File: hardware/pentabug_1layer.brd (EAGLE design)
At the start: 33 x 82.9 mm, 17 parts, among them IC1 ATMEGA88

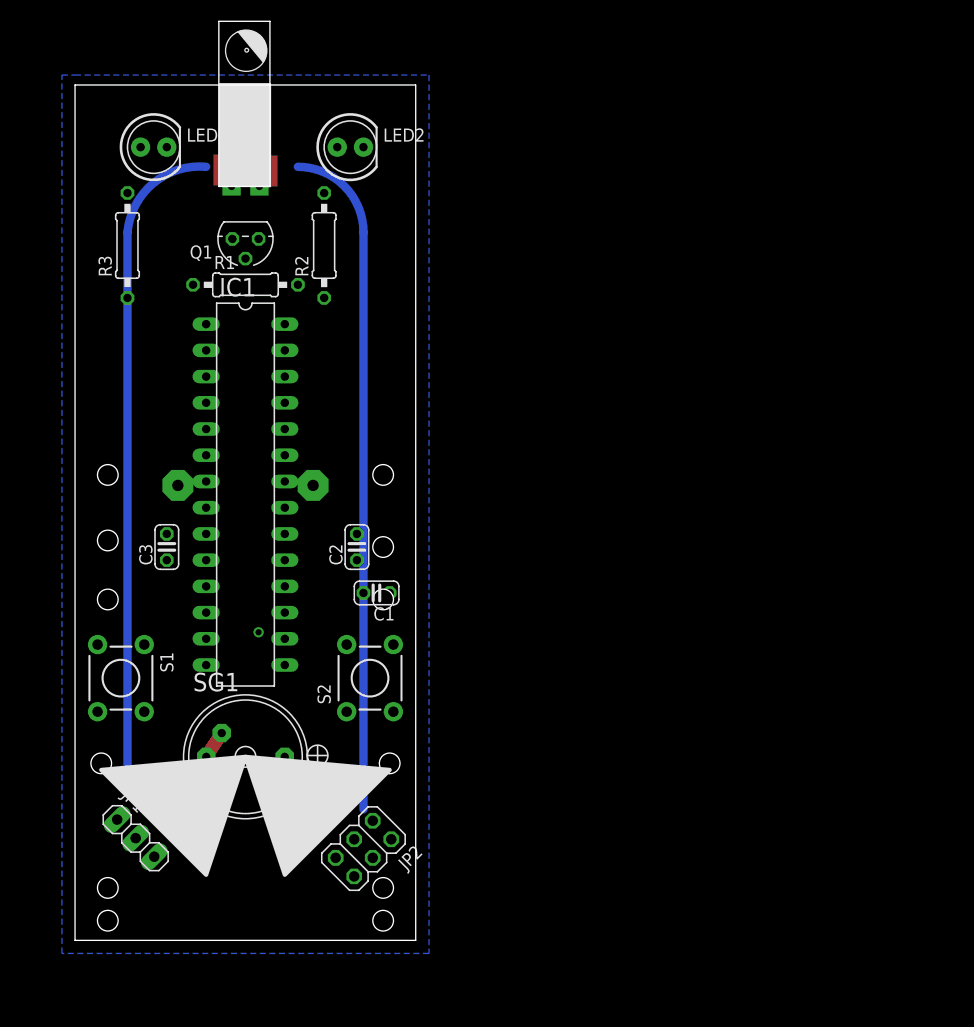
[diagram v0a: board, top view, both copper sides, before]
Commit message: made editable with eagle freeware!!
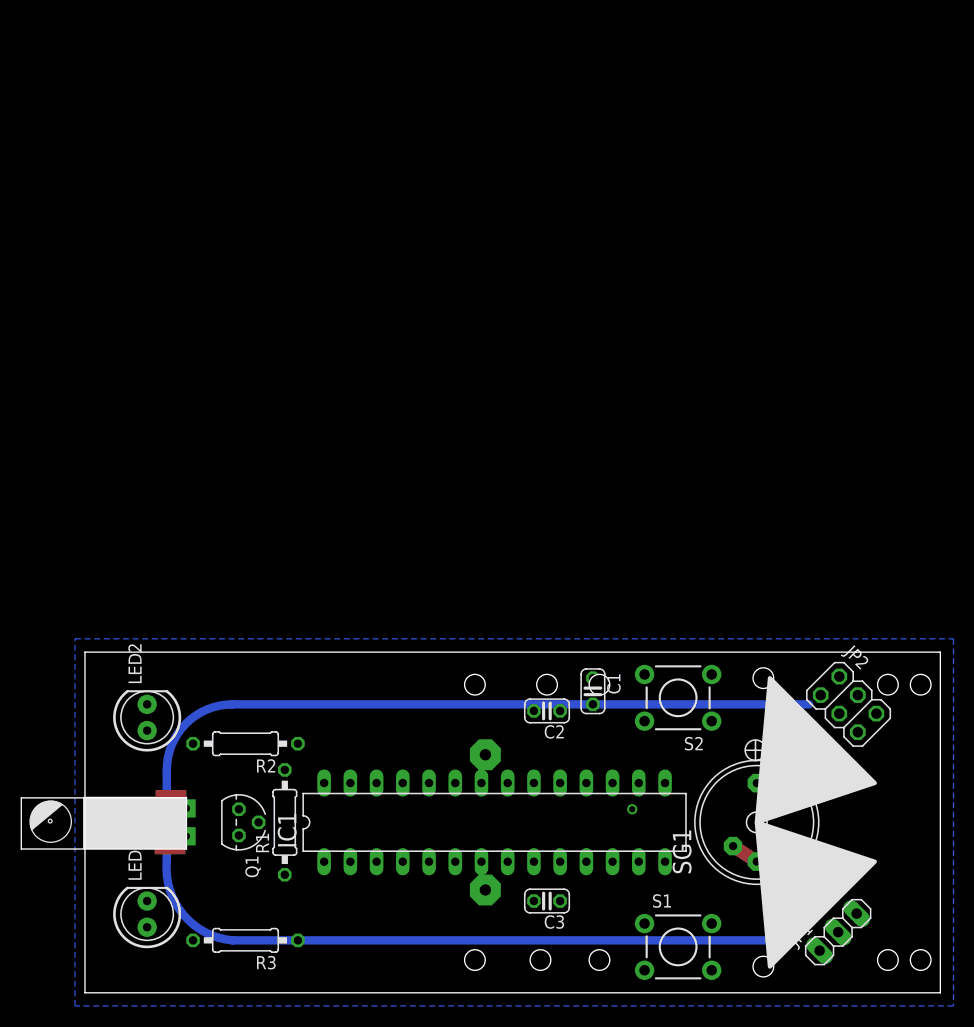
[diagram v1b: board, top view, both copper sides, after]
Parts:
- moved LED1 74.3 mm to (6.99, 8.89), turned to 90 degrees
- moved U$1 69.7 mm to (3.81, 17.8), turned to 180 degrees
- moved JP1 68.6 mm to (73.9, 7.15), turned to 45 degrees
- moved R3 68.3 mm to (16.5, 6.35), turned to 180 degrees
- moved S1 59.9 mm to (58.4, 5.71), turned to 0 degrees
- moved LED2 58.6 mm to (6.99, 27.9), turned to 90 degrees
- moved Q1 56.5 mm to (15.9, 17.8), turned to 270 degrees
- moved R1 52.2 mm to (20.3, 17.8), turned to 90 degrees
- moved C3 50.3 mm to (45.7, 10.2), turned to 180 degrees
- moved SG1 49.9 mm to (66.0, 17.8), turned to 90 degrees
- moved JP2 49.0 mm to (74.9, 29.2), turned to 315 degrees
- moved R2 48.9 mm to (16.5, 25.4), turned to 180 degrees
- moved BAT1 47.8 mm to (63.5, 17.8), turned to 180 degrees
- moved IC1 39.9 mm to (40.6, 17.8), turned to 0 degrees
- moved S2 29.9 mm to (58.4, 29.8), turned to 180 degrees
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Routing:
- net VCC: track 0.00 -> 137.0 mm
- net N$2: track 64.9 -> 0.00 mm
- net N$1: track 63.3 -> 0.00 mm
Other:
- board size 33 x 82.9 mm -> 82.9 x 33 mm
